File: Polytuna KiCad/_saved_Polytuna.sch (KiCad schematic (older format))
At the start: 43 parts, among them IC1 AP7313-33SAG-7, J1 Barrel_Jack, J2 Conn_01x02, J3 Conn_01x02, J4 Conn_01x04, SW1 SW_Push, SW2 SW_Push, SW3 SW_Push, SW4 SW_DPDT_x2, U1 LM358, U2 SGTL5000, U3 L7805

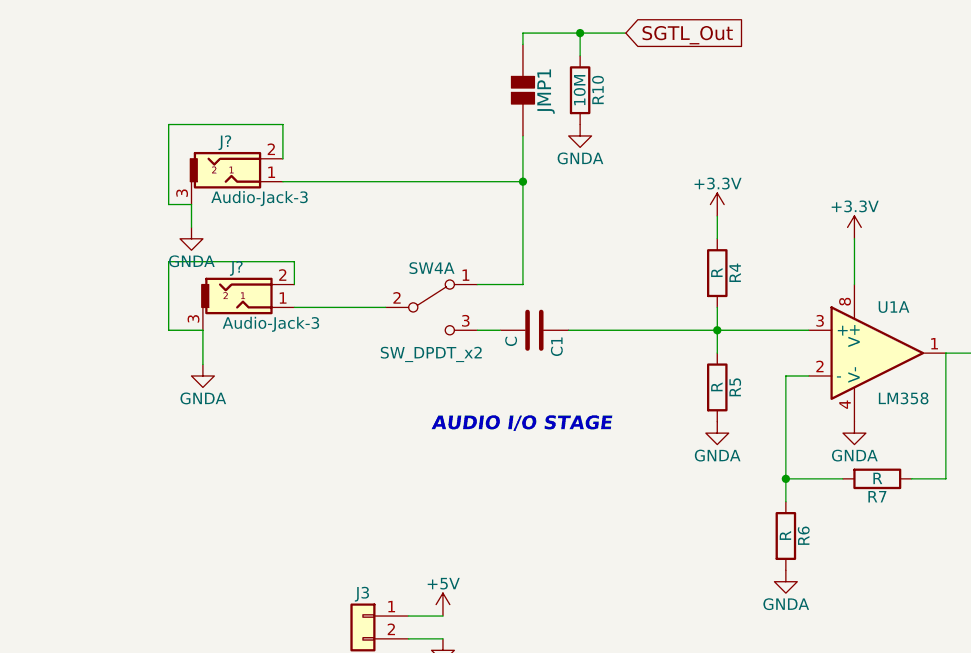
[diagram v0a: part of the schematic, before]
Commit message: Moar routing x2
Still have to add the 3pdt
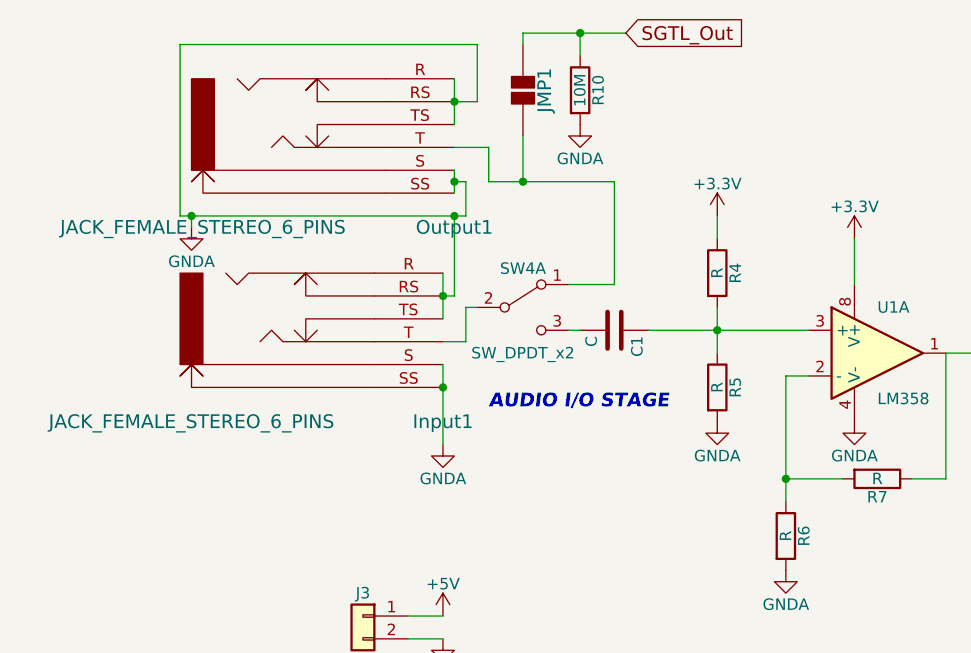
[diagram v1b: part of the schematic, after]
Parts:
- removed J?: Audio-Jack-3, symbol Audio-Jack-3
- removed J?: Audio-Jack-3, def-footprints:CONN_Jack_Female_6.35mm_THD, symbol Audio-Jack-3
- added Input1, Output1: JACK_FEMALE_STEREO_6_PINS, def-footprints:CONN_Jack_Female_6.35mm_THD, symbol JACK_FEMALE_STEREO_6_PINS
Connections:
- net GNDA: now also Input1.R, Input1.RS, Input1.S, Input1.SS, Input1.TS, Output1.R, Output1.RS, Output1.S, Output1.SS, Output1.TS
- net at JMP1.2, SW4.1 (A): now also Output1.T
- net at SW4.2 (B): now also Input1.T
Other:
- moved on the sheet: C1, SW4A
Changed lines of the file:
@@
 LIBS:ws2812b
 LIBS:AP7313-33SAG-7
+LIBS:dynamixel_conn_3
+LIBS:jack_female_mono
+LIBS:jack_female_mono_3_pins
+LIBS:jack_female_stereo_3_pins
+LIBS:jack_female_stereo_5_pins
+LIBS:jack_female_stereo_6_pins
+LIBS:usb-female
 LIBS:Polytuna-cache
 EELAYER 25 0
@@
 L C C1
 U 1 1 5A947E19
-P 2100 1850
-F 0 "C1" H 2125 1950 50  0000 L CNN
-F 1 "C" H 2125 1750 50  0000 L CNN
-F 2 "Capacitors_SMD:C_0805" H 2138 1700 50  0001 C CNN
-F 3 "" H 2100 1850 50  0001 C CNN
-	1    2100 1850
+P 2450 1850
+F 0 "C1" H 2475 1950 50  0000 L CNN
+F 1 "C" H 2475 1750 50  0000 L CNN
+F 2 "Capacitors_SMD:C_0805" H 2488 1700 50  0001 C CNN
+F 3 "" H 2450 1850 50  0001 C CNN
+	1    2450 1850
 	0    1    1    0
 $EndComp
@@
 L SW_DPDT_x2 SW4
 U 1 1 5A99587A
-P 1650 1750
-F 0 "SW4" H 1650 1920 50  0000 C CNN
-F 1 "SW_DPDT_x2" H 1650 1550 50  0000 C CNN
-F 2 "def-footprints:Switches_Stomp_Switch_3PDT" H 1650 1750 50  0001 C CNN
-F 3 "" H 1650 1750 50  0001 C CNN
-	1    1650 1750
+P 2050 1750
+F 0 "SW4" H 2050 1920 50  0000 C CNN
+F 1 "SW_DPDT_x2" H 2050 1550 50  0000 C CNN
+F 2 "def-footprints:Switches_Stomp_Switch_3PDT" H 2050 1750 50  0001 C CNN
+F 3 "" H 2050 1750 50  0001 C CNN
+	1    2050 1750
 	1    0    0    -1
 $EndComp
@@
 $EndComp
 Wire Wire Line
-	2250 1850 3300 1850
+	2600 1850 3300 1850
 Wire Wire Line
 	3200 2050 3200 2600
@@
 Connection ~ 3200 2500
 Wire Wire Line
-	1850 1850 1950 1850
-Wire Wire Line
-	2050 1650 1850 1650
-Wire Wire Line
-	2050 1000 2050 1650
-Wire Wire Line
-	1000 1200 2050 1200
+	2250 1850 2300 1850
+Wire Wire Line
+	2450 1650 2250 1650
 Wire Wire Line
 	7550 3650 8650 3650
@@
 Text Notes 5000 3400 0    60   Italic 12
 POWER STAGE
-Text Notes 1650 2300 0    60   Italic 12
+Text Notes 1900 2200 0    60   Italic 12
 AUDIO I/O STAGE
 Text Notes 750  7150 0    60   Italic 12
@@
 L GNDA #PWR043
 U 1 1 5AA2CADA
-P 650 2000
-F 0 "#PWR043" H 650 1750 50  0001 C CNN
-F 1 "GNDA" H 650 1850 50  0000 C CNN
-F 2 "" H 650 2000 50  0001 C CNN
-F 3 "" H 650 2000 50  0001 C CNN
-	1    650  2000
+P 1700 2350
+F 0 "#PWR043" H 1700 2100 50  0001 C CNN
+F 1 "GNDA" H 1700 2200 50  0000 C CNN
+F 2 "" H 1700 2350 50  0001 C CNN
+F 3 "" H 1700 2350 50  0001 C CNN
+	1    1700 2350
 	1    0    0    -1
 $EndComp
@@
 NoConn ~ 2700 5650
 $Comp
-L GND #PWR?
+L GND #PWR052
 U 1 1 5AABFC35
 P 9750 4400
-F 0 "#PWR?" H 9750 4150 50  0001 C CNN
+F 0 "#PWR052" H 9750 4150 50  0001 C CNN
 F 1 "GND" H 9750 4250 50  0000 C CNN
 F 2 "" H 9750 4400 50  0001 C CNN
@@
 $EndComp
 $Comp
-L Audio-Jack-3 J?
-U 1 1 5AAD6F13
-P 800 1200
-F 0 "J?" H 750 1375 50  0000 C CNN
-F 1 "Audio-Jack-3" H 900 1130 50  0000 C CNN
-F 2 "" H 1050 1300 50  0001 C CNN
-F 3 "" H 1050 1300 50  0001 C CNN
-	1    800  1200
-	1    0    0    -1
-$EndComp
-$Comp
-L Audio-Jack-3 J?
-U 1 1 5AAD73D6
-P 850 1750
-F 0 "J?" H 800 1925 50  0000 C CNN
-F 1 "Audio-Jack-3" H 950 1680 50  0000 C CNN
-F 2 "def-footprints:CONN_Jack_Female_6.35mm_THD" H 1100 1850 50  0001 C CNN
-F 3 "" H 1100 1850 50  0001 C CNN
-	1    850  1750
-	1    0    0    -1
-$EndComp
+L JACK_FEMALE_STEREO_6_PINS Output1
+U 1 1 5AADD4DA
+P 1200 900
+F 0 "Output1" H 1750 400 60  0000 C CNN
+F 1 "JACK_FEMALE_STEREO_6_PINS" H 650 400 60  0000 C CNN
+F 2 "def-footprints:CONN_Jack_Female_6.35mm_THD" H 1650 850 60  0001 C CNN
+F 3 "" H 1650 850 60  0000 C CNN
+	1    1200 900
+	1    0    0    -1
+$EndComp
+Wire Wire Line
+	1750 750  1750 950
+Wire Wire Line
+	1750 1150 1750 1250
+Connection ~ 1750 850
+Wire Wire Line
+	1750 1050 1900 1050
+Wire Wire Line
+	1900 1050 1900 1200
+Wire Wire Line
+	1750 1200 1800 1200
+Wire Wire Line
+	1800 1200 1800 1350
+Wire Wire Line
+	1800 1350 550  1350
+Wire Wire Line
+	600  1350 600  1400
+Connection ~ 1750 1200
+Wire Wire Line
+	1750 850  1850 850
+Wire Wire Line
+	1850 850  1850 600
+Wire Wire Line
+	1850 600  550  600
+Wire Wire Line
+	550  600  550  1350
+Connection ~ 600  1350
+$Comp
+L JACK_FEMALE_STEREO_6_PINS Input1
+U 1 1 5AADE263
+P 1150 1750
+F 0 "Input1" H 1700 1250 60  0000 C CNN
+F 1 "JACK_FEMALE_STEREO_6_PINS" H 600 1250 60  0000 C CNN
+F 2 "def-footprints:CONN_Jack_Female_6.35mm_THD" H 1600 1700 60  0001 C CNN
+F 3 "" H 1600 1700 60  0000 C CNN
+	1    1150 1750
+	1    0    0    -1
+$EndComp
+Wire Wire Line
+	2450 1200 2450 1650
+Wire Wire Line
+	1900 1200 2450 1200
+Wire Wire Line
+	2050 1000 2050 1200
 Connection ~ 2050 1200
 Wire Wire Line
-	1000 1100 1000 950
-Wire Wire Line
-	1000 950  500  950
-Wire Wire Line
-	500  950  500  1300
-Wire Wire Line
-	500  1300 600  1300
-Wire Wire Line
-	600  1300 600  1400
-Wire Wire Line
-	1050 1750 1450 1750
-Wire Wire Line
-	1050 1650 1050 1550
-Wire Wire Line
-	1050 1550 500  1550
-Wire Wire Line
-	500  1550 500  1850
-Wire Wire Line
-	500  1850 650  1850
-Wire Wire Line
-	650  1850 650  2000
+	1700 1900 1800 1900
+Wire Wire Line
+	1800 1900 1800 1750
+Wire Wire Line
+	1800 1750 1850 1750
+Wire Wire Line
+	1700 1600 1700 1800
+Connection ~ 1700 1700
+Wire Wire Line
+	1700 1700 1750 1700
+Wire Wire Line
+	1750 1700 1750 1350
+Connection ~ 1750 1350
+Wire Wire Line
+	1700 2000 1700 2350
+Connection ~ 1700 2100
 $EndSCHEMATC
